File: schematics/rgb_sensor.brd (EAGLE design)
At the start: 67 x 40.6 mm, 7 parts, among them IC2 MEGA8-P

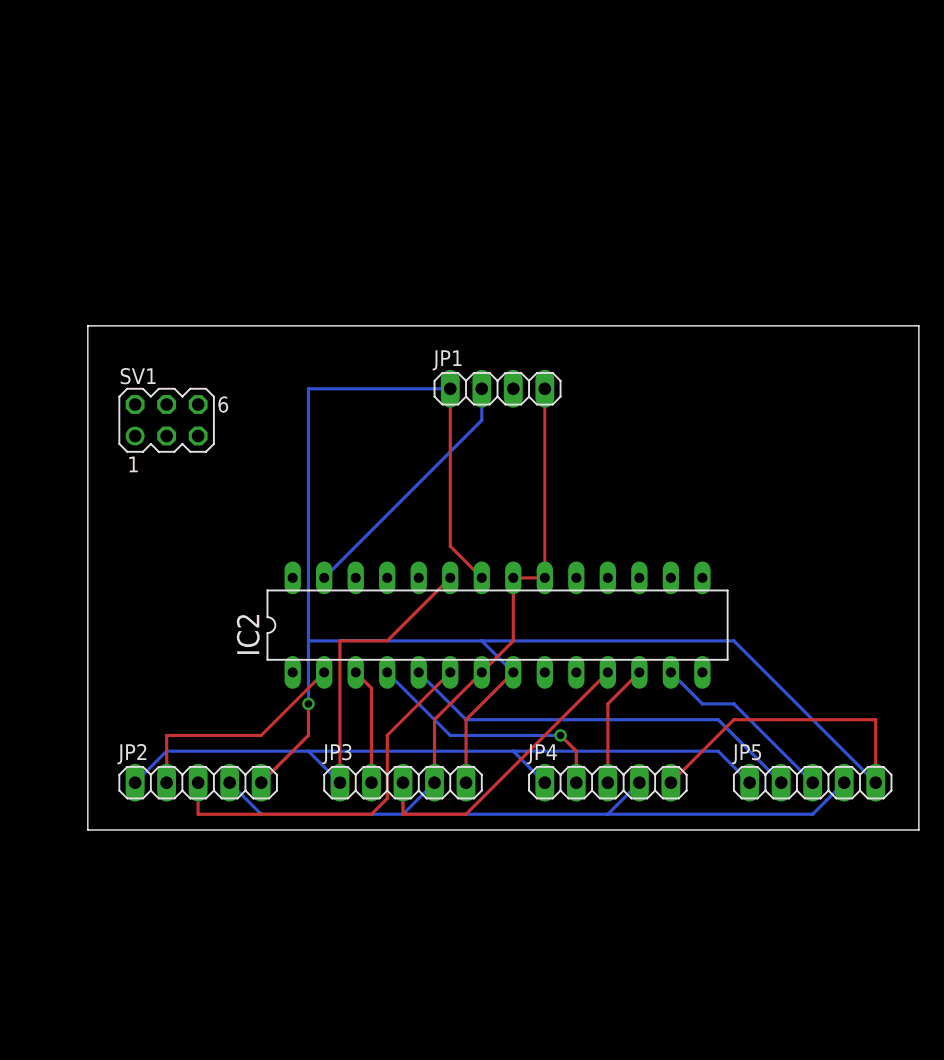
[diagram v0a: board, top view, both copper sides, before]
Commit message: RGB Color Sensor Array Board Finalized to be Printed
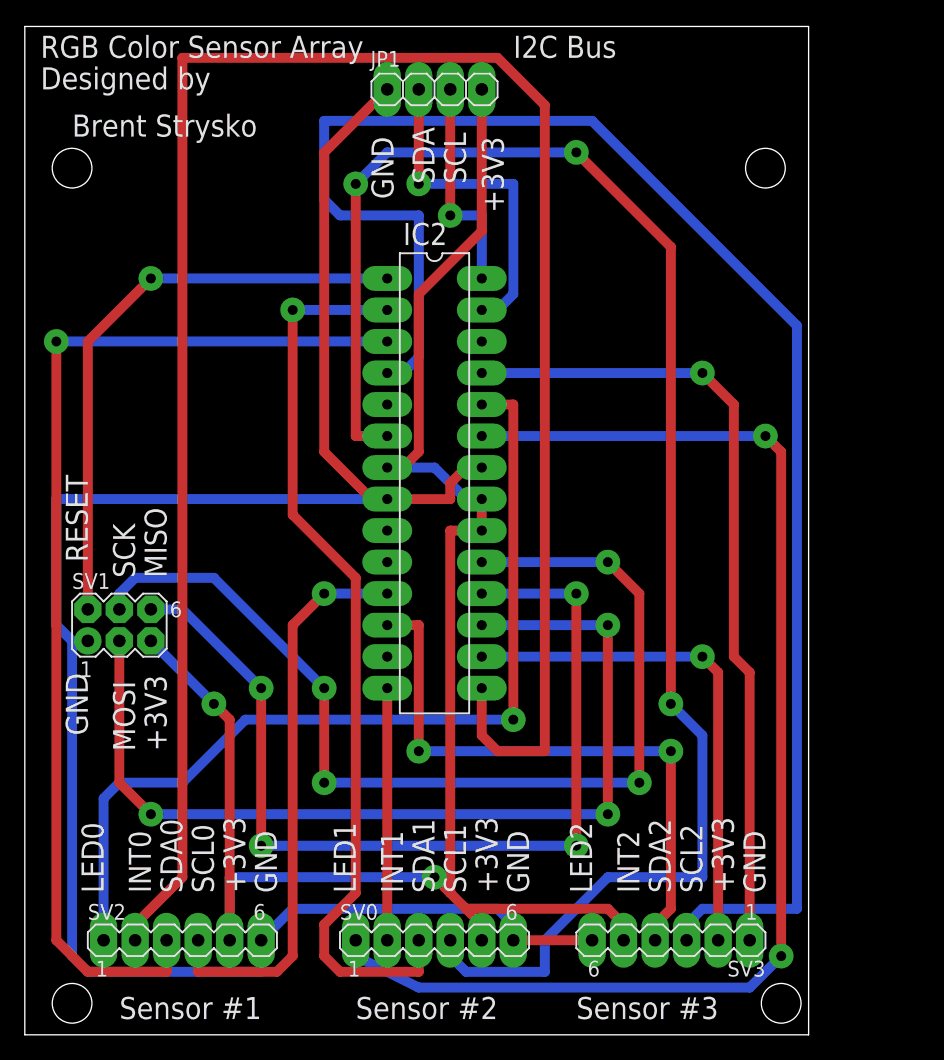
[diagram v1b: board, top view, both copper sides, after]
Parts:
- removed JP2: RGBSENSOR0, pinhead:1X05
- removed JP3: RGBSENSOR1, pinhead:1X05
- removed JP4: RGBSENSOR2, pinhead:1X05
- removed JP5: RGBSENSOR3, pinhead:1X05
- added SV0, SV2, SV3: (no value), con-lstb:MA06-1
- moved JP1 24.7 mm to (44.5, 74.9)
- moved SV1 16.9 mm to (19.1, 31.8)
- moved IC2 12.5 mm to (44.5, 43.2), turned to 270 degrees
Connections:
- removed net BBB_SDL: IC2.28
- removed net LED3: IC2.26
- removed net SCL3: IC2.13, JP5.3
- removed net SDA3: IC2.5, JP5.2
- new net INT0: IC2.14, SV0.2
- new net INT1: IC2.15, SV2.2
- new net INT2: IC2.16, SV3.2
- net +3V3: now also SV0.5, SV1.5, SV2.5, SV3.5; no longer JP2.4, JP3.4, JP4.4, JP5.4
- net BBB_SCL: now also IC2.28
- net GND: now also SV0.6, SV1.1, SV2.6, SV3.6; no longer JP2.5, JP3.5, JP4.5, JP5.5
- net LED0: now also SV0.1; no longer JP2.1, JP3.1, JP4.1, JP5.1
- net LED1: now also SV2.1
- net LED2: now also SV3.1
- net MISO: now also SV1.6
- net MOSI: now also SV1.3
- net RESET: now also SV1.2
- net SCK: now also SV1.4
- net SCL0: now also SV0.4; no longer JP2.3
- net SCL1: now also SV2.4; no longer JP3.3
- net SCL2: now also SV3.4; no longer JP4.3
- net SDA0: now also SV0.3; no longer JP2.2
- net SDA1: now also SV2.3; no longer JP3.2
- net SDA2: now also SV3.3; no longer JP4.2
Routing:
- net INT1: track 0.00 -> 165.0 mm
- net SDA2: track 20.4 -> 131.6 mm, vias 1 -> 0
- net SCL0: track 30.6 -> 131.1 mm, vias 0 -> 3
- net SCK: track 0.00 -> 84.0 mm, vias 0 -> 4
- net SDA1: track 9.42 -> 87.4 mm, vias 0 -> 1
- net MISO: track 0.00 -> 77.6 mm, vias 0 -> 4
- net MOSI: track 0.00 -> 77.3 mm, vias 0 -> 3
- net LED1: track 0.00 -> 75.0 mm, vias 0 -> 1
- net LED2: track 0.00 -> 65.1 mm, vias 0 -> 1
- net SDA0: track 18.6 -> 73.5 mm, vias 0 -> 1
- net +3V3: track 95.7 -> 146.8 mm, vias 0 -> 2
- net RESET: track 0.00 -> 47.8 mm, vias 0 -> 1
- net INT2: track 0.00 -> 41.2 mm, vias 0 -> 1
- net SCL2: track 9.94 -> 48.8 mm, vias 0 -> 2
- net SDA3: track 32.9 -> 0.00 mm
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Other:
- board size 67 x 40.6 mm -> 63.2 x 81.3 mm
- board text added: "+3V3"
- board text added: "Brent Strysko"
- board text added: "Designed by"
- board text added: "GND"
- board text added: "I2C Bus"
- board text added: "INT0"
- board text added: "INT1"
- board text added: "INT2"
- board text added: "LED0"
- board text added: "LED1"
- board text added: "LED2"
- board text added: "MISO"
- board text added: "MOSI"
- board text added: "RESET"
- board text added: "RGB Color Sensor Array"
- board text added: "SCK"
- board text added: "SCL"
- board text added: "SCL0"
- board text added: "SCL1"
- board text added: "SCL2"
- board text added: "SDA"
- board text added: "SDA0"
- board text added: "SDA1"
- board text added: "SDA2"
- board text added: "Sensor #1"
- board text added: "Sensor #2"
- board text added: "Sensor #3"
